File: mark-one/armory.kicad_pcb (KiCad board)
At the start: 8 copper layers, 65.6 x 19.6 mm, 184 parts, among them J1 MICRO_SD_HINGE, J2 USB_A_PLUG, P1 TST, P10 TST, P11 TST, P12 TST, P13 TST, P2 TST, P3 TST, P4 CONN_01X07, P5 TST, P6 TST, P8 TST, P9 TST, U2 MX53, U3 NCP1529, U4 MT41K256M16HA, U5 TPD2E001DRLR, X1 32.768kHz, X2 24MHz

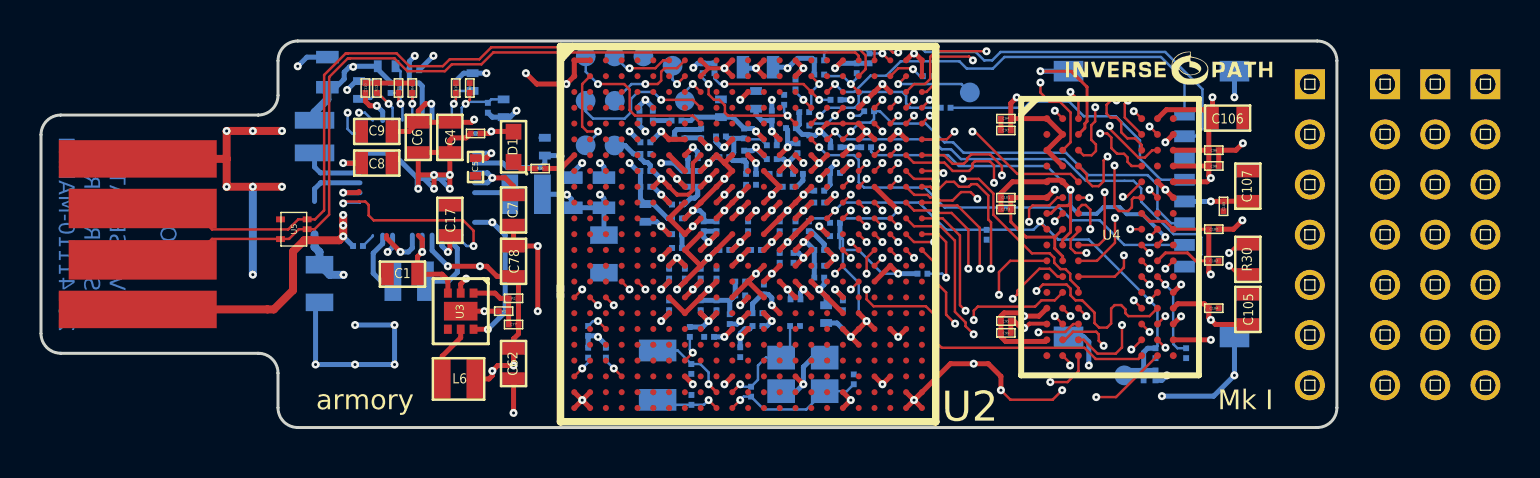
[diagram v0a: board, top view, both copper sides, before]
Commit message: added zones again
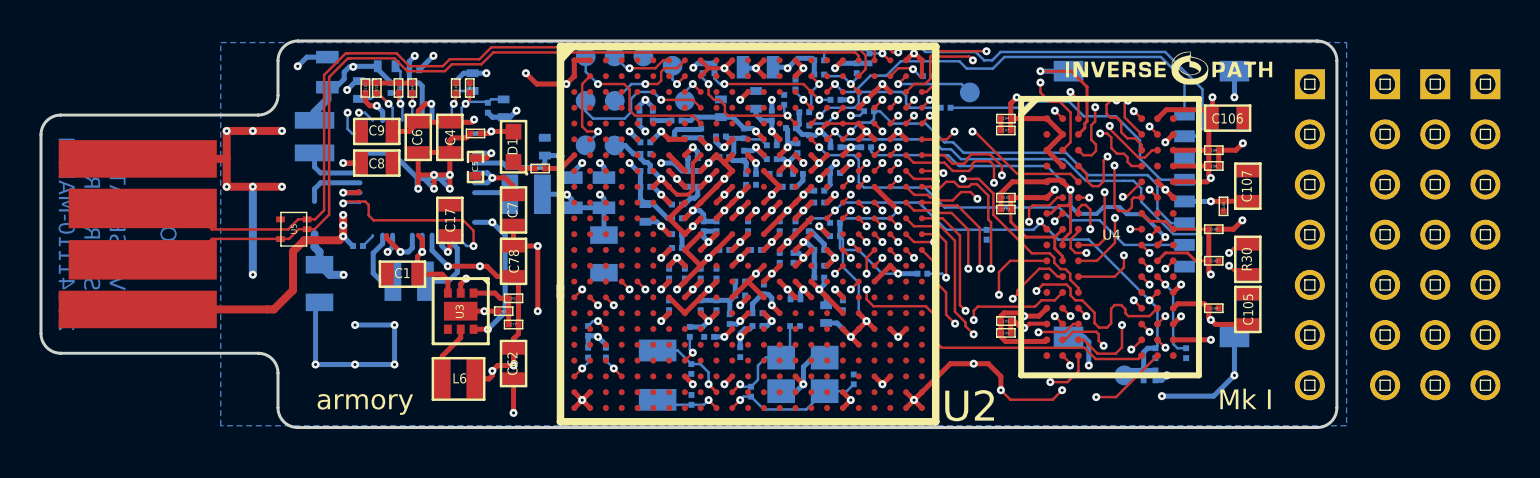
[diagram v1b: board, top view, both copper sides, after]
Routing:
- added copper zone on GND_POWER_2, net /Interfaces/USB_VBUS
- added copper zone on B.Cu, net GND
- added copper zone on SIGNAL_2, net GND
- added copper zone on GND_POWER_1, net IMX53_LDO_1V8
- added copper zone on GND_POWER_2, net PMIC_DDR_1V5
- added copper zone on GND_POWER_1, net PMIC_LDO1_STDBY
- added copper zone on GND_POWER_2, net PMIC_SW1_VDDGP
- added copper zone on GND_POWER_1, net PMIC_SW2_VCC
- added copper zone on GND_POWER_1, net PMIC_SW3_2V5
- added copper zone on GND_POWER_2, net PMIC_SW4_3V3
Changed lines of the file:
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@@
   (layers
     (0 TOP signal)
-    (1 GND_1 power)
+    (1 GND_1 power hide)
     (2 SIGNAL_1 signal)
-    (3 GND_POWER_1 power)
-    (4 GND_POWER_2 power)
-    (5 SIGNAL_2 signal)
-    (6 GND_2 power)
-    (31 BOTTOM signal)
+    (3 GND_POWER_1 power hide)
+    (4 GND_POWER_2 power hide)
+    (5 SIGNAL_2 signal hide)
+    (6 GND_2 power hide)
+    (31 BOTTOM signal hide)
     (32 B.Adhes user)
     (33 F.Adhes user)
@@
   (segment (start 130.425 92.075) (end 129.625 92.075) (width 0.254) (layer TOP) (net 126))
   (segment (start 131.1 91.4) (end 130.425 92.075) (width 0.254) (layer TOP) (net 126))
+  (zone (net 1) (net_name GND) (layer BOTTOM) (hatch edge 0.508)
+    (connect_pads (clearance 0.25))
+    (min_thickness 0.127)
+    (fill (arc_segments 16) (thermal_gap 0.254) (thermal_bridge_width 0.4064))
+    (polygon
+      (pts
+        (xy 170.2 105.1) (xy 113.2 105.1) (xy 113.2 85.7) (xy 170.2 85.7)
+      )
+    )
+  )
+  (zone (net 1) (net_name GND) (layer SIGNAL_2) (hatch edge 0.508)
+    (connect_pads (clearance 0.127))
+    (min_thickness 0.127)
+    (fill (arc_segments 16) (thermal_gap 0.254) (thermal_bridge_width 0.4064))
+    (polygon
+      (pts
+        (xy 170.2 105.1) (xy 104 105.1) (xy 104 85.7) (xy 170.2 85.7)
+      )
+    )
+  )
+  (zone (net 55) (net_name PMIC_SW4_3V3) (layer GND_POWER_2) (hatch edge 0.508)
+    (connect_pads (clearance 0.127))
+    (min_thickness 0.127)
+    (fill (arc_segments 16) (thermal_gap 0.254) (thermal_bridge_width 0.4064))
+    (polygon
+      (pts
+        (xy 139.7 99.2) (xy 138.7 99.2) (xy 138.7 100.1) (xy 133.1 100.1) (xy 133.1 101)
+        (xy 131.4 101) (xy 117.45 101) (xy 117.45 88.6) (xy 121.3 88.6) (xy 121.3 90.75)
+        (xy 118.4 90.75) (xy 118.4 96.05) (xy 122.6 96.05) (xy 122.6 99) (xy 125 99)
+        (xy 130.725 99) (xy 130.725 97.6) (xy 135.2 97.6) (xy 135.2 96.3) (xy 135.8 96.3)
+        (xy 135.8 98.7) (xy 139.7 98.7)
+      )
+    )
+  )
+  (zone (net 59) (net_name PMIC_DDR_1V5) (layer GND_POWER_2) (hatch edge 0.508)
+    (connect_pads (clearance 0.127))
+    (min_thickness 0.127)
+    (fill (arc_segments 16) (thermal_gap 0.254) (thermal_bridge_width 0.4064))
+    (polygon
+      (pts
+        (xy 146.45 104.05) (xy 124.6 104.05) (xy 124.6 101.85) (xy 144.1 101.85) (xy 144.1 92.5)
+        (xy 144.8 92.5) (xy 144.8 91.5) (xy 144.8 88.23) (xy 164.05 88.23) (xy 164.05 104.05)
+      )
+    )
+  )
+  (zone (net 58) (net_name PMIC_SW2_VCC) (layer GND_POWER_1) (hatch edge 0.508)
+    (connect_pads (clearance 0.127))
+    (min_thickness 0.127)
+    (fill (arc_segments 16) (thermal_gap 0.254) (thermal_bridge_width 0.4064))
+    (polygon
+      (pts
+        (xy 143.9 98.5) (xy 136 98.5) (xy 136 97.8) (xy 119.1 97.8) (xy 119.1 94.45)
+        (xy 119.7 94.45) (xy 119.7 91.05) (xy 118.775 91.05) (xy 118.775 87.65) (xy 119.95 87.65)
+        (xy 119.95 88.1) (xy 120.35 88.1) (xy 120.35 93.6) (xy 120.2 93.6) (xy 120.2 96.5)
+        (xy 119.75 96.5) (xy 119.75 97) (xy 123.05 97) (xy 123.05 96.525) (xy 124.35 96.525)
+        (xy 124.35 95.2) (xy 125.3 95.2) (xy 125.3 97) (xy 136 97) (xy 136 96.3)
+        (xy 140.8 96.3) (xy 140.8 93.2) (xy 143 93.2) (xy 143 97.4) (xy 143.9 97.4)
+        (xy 143.9 98.5)
+      )
+    )
+  )
+  (zone (net 60) (net_name IMX53_LDO_1V8) (layer GND_POWER_1) (hatch edge 0.508)
+    (connect_pads (clearance 0.127))
+    (min_thickness 0.127)
+    (fill (arc_segments 16) (thermal_gap 0.254) (thermal_bridge_width 0.4064))
+    (polygon
+      (pts
+        (xy 143.7 92.75) (xy 140.3 92.75) (xy 140.3 95.35) (xy 125.8 95.35) (xy 125.8 94.7)
+        (xy 122.1 94.7) (xy 122.1 96.5) (xy 120.7 96.5) (xy 120.7 94.1) (xy 125.8 94.1)
+        (xy 125.8 93.25) (xy 138.7 93.25) (xy 138.7 92.5) (xy 142.6 92.5) (xy 142.6 91.6)
+        (xy 143.7 91.6)
+      )
+    )
+  )
   (zone (net 54) (net_name PMIC_LDO3_2V8) (layer GND_POWER_1) (hatch edge 0.508)
     (connect_pads (clearance 0.127))
@@
     )
   )
+  (zone (net 53) (net_name PMIC_LDO1_STDBY) (layer GND_POWER_1) (hatch edge 0.508)
+    (connect_pads (clearance 0.127))
+    (min_thickness 0.127)
+    (fill (arc_segments 16) (thermal_gap 0.254) (thermal_bridge_width 0.4064))
+    (polygon
+      (pts
+        (xy 138.925 100.9) (xy 133.3 100.9) (xy 133.3 101.9) (xy 131.1 101.9) (xy 117.4 101.9)
+        (xy 117.4 85.75) (xy 123.25 85.75) (xy 123.25 86.65) (xy 122.8 86.65) (xy 122.8 86.2)
+        (xy 118.3 86.2) (xy 118.3 100.3) (xy 138.925 100.3)
+      )
+    )
+  )
   (zone (net 110) (net_name IMX53_LDO_1V3) (layer GND_POWER_2) (hatch edge 0.508)
     (connect_pads (clearance 0.127))
@@
     )
   )
+  (zone (net 119) (net_name /Interfaces/USB_VBUS) (layer GND_POWER_2) (hatch edge 0.508)
+    (connect_pads (clearance 0.127))
+    (min_thickness 0.127)
+    (fill (arc_segments 16) (thermal_gap 0.127) (thermal_bridge_width 0.4064))
+    (polygon
+      (pts
+        (xy 169.4 91.4) (xy 166.15 91.4) (xy 166.15 87.75) (xy 144.8 87.75) (xy 144.8 86.4)
+        (xy 138.425 86.4) (xy 138.425 87.4) (xy 136.8 87.4) (xy 136.8 86.4) (xy 125.3 86.4)
+        (xy 125.3 88.225) (xy 127.2 88.225) (xy 127.2 90.55) (xy 126.25 90.55) (xy 126.25 92)
+        (xy 127.2 92) (xy 127.2 94.1) (xy 124.2 94.1) (xy 124.2 96.6) (xy 123.175 96.6)
+        (xy 123.175 95.575) (xy 119.1 95.575) (xy 119.1 95.075) (xy 119.1 91.4) (xy 123 91.4)
+        (xy 123 85.8) (xy 169.4 85.8)
+      )
+    )
+  )
+  (zone (net 57) (net_name PMIC_SW1_VDDGP) (layer GND_POWER_2) (hatch edge 0.508)
+    (connect_pads (clearance 0.127))
+    (min_thickness 0.254)
+    (fill (arc_segments 16) (thermal_gap 0.508) (thermal_bridge_width 0.508))
+    (polygon
+      (pts
+        (xy 140.6 94.4) (xy 129.675 94.4) (xy 129.675 88.3) (xy 127.8 88.3) (xy 127.8 87.725)
+        (xy 126.375 87.725) (xy 126.375 86.9) (xy 130.825 86.9) (xy 130.825 90.7) (xy 137.3 90.7)
+        (xy 137.3 91.6) (xy 138.95 91.6) (xy 138.95 93.1) (xy 140.6 93.1)
+      )
+    )
+  )
   (zone (net 60) (net_name IMX53_LDO_1V8) (layer GND_POWER_2) (hatch edge 0.508)
     (connect_pads (clearance 0.127))
@@
       )
     )
+  )
+  (zone (net 56) (net_name PMIC_SW3_2V5) (layer GND_POWER_1) (hatch edge 0.508)
+    (connect_pads (clearance 0.127))
+    (min_thickness 0.127)
+    (fill (arc_segments 16) (thermal_gap 0.254) (thermal_bridge_width 0.4064))
+    (polygon
+      (pts
+        (xy 146.7 100.9) (xy 140.875 100.9) (xy 140.875 99.35) (xy 144.5 99.35) (xy 144.5 90.5)
+        (xy 145.9 90.5) (xy 145.9 87.9) (xy 135.9 87.9) (xy 135.9 89.2) (xy 133.5 89.2)
+        (xy 133.5 87.9) (xy 120.85 87.9) (xy 120.85 87.3) (xy 119.6 87.3) (xy 119.6 86.7)
+        (xy 122.2 86.7) (xy 122.2 87.15) (xy 123.9 87.15) (xy 123.9 85.75) (xy 146.7 85.75)
+      )
+    )
+  )
+  (zone (net 55) (net_name PMIC_SW4_3V3) (layer GND_POWER_1) (hatch edge 0.508)
+    (connect_pads (clearance 0.127))
+    (min_thickness 0.127)
+    (fill (arc_segments 16) (thermal_gap 0.254) (thermal_bridge_width 0.4064))
+    (polygon
+      (pts
+        (xy 164.125 104.875) (xy 139.725 104.875) (xy 139.725 99.5) (xy 139.275 99.5) (xy 139.275 98.775)
+        (xy 140.3 98.775) (xy 140.3 103.875) (xy 163.275 103.875) (xy 163.275 94.3) (xy 161.675 94.3)
+        (xy 161.675 93.275) (xy 164.125 93.275)
+      )
+    )
+  )
+  (zone (net 1) (net_name GND) (layer GND_POWER_1) (hatch edge 0.508)
+    (connect_pads (clearance 0.127))
+    (min_thickness 0.127)
+    (fill (arc_segments 16) (thermal_gap 0.254) (thermal_bridge_width 0.4064))
+    (polygon
+      (pts
+        (xy 164.625 92.775) (xy 161.175 92.775) (xy 161.175 94.8) (xy 162.775 94.8) (xy 162.775 103.375)
+        (xy 147.2 103.375) (xy 147.2 85.75) (xy 164.625 85.75)
+      )
+    )
+  )
+  (zone (net 59) (net_name PMIC_DDR_1V5) (layer GND_POWER_2) (hatch edge 0.508)
+    (connect_pads (clearance 0.127))
+    (min_thickness 0.127)
+    (fill (arc_segments 16) (thermal_gap 0.254) (thermal_bridge_width 0.4064))
+    (polygon
+      (pts
+        (xy 129.675 98.5) (xy 125.975 98.5) (xy 125.975 96.325) (xy 126.925 96.325) (xy 126.925 94.975)
+        (xy 127.75 94.975) (xy 127.75 89.65) (xy 129.175 89.65) (xy 129.175 94.975) (xy 129.675 94.975)
+      )
+    )

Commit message: removed zones
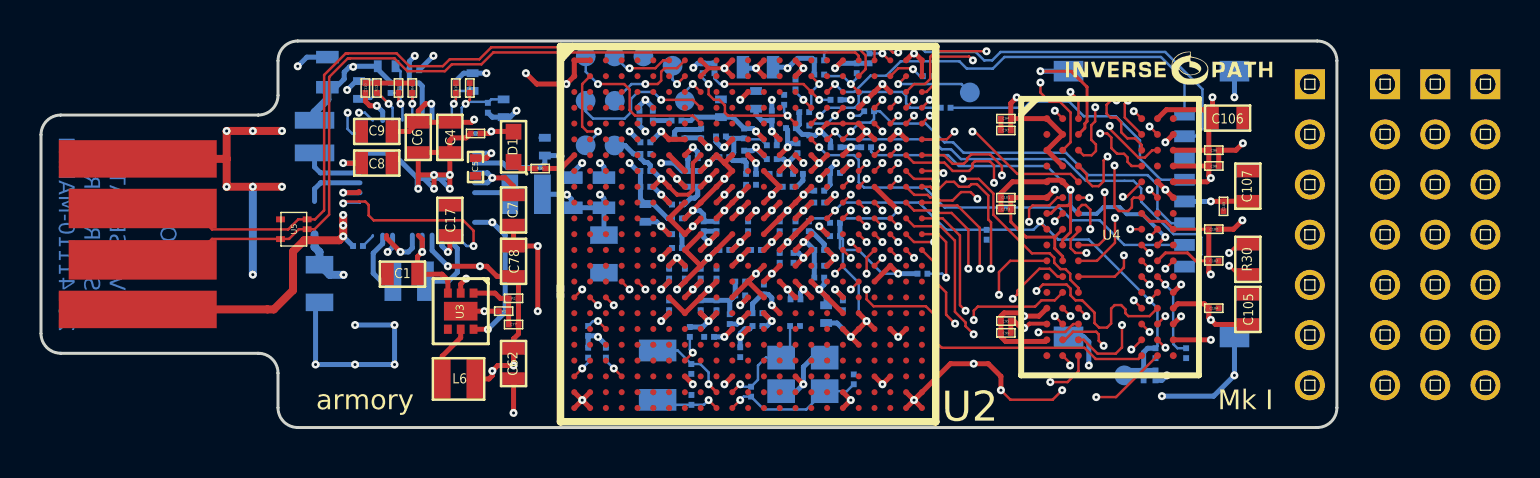
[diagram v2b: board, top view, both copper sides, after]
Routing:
- removed copper zone on GND_POWER_2, net /Interfaces/USB_VBUS
- removed copper zone on B.Cu, net GND
- removed copper zone on SIGNAL_2, net GND
- removed copper zone on GND_POWER_1, net IMX53_LDO_1V8
- removed copper zone on GND_POWER_2, net PMIC_DDR_1V5
- removed copper zone on GND_POWER_1, net PMIC_LDO1_STDBY
- removed copper zone on GND_POWER_2, net PMIC_SW1_VDDGP
- removed copper zone on GND_POWER_1, net PMIC_SW2_VCC
- removed copper zone on GND_POWER_1, net PMIC_SW3_2V5
- removed copper zone on GND_POWER_2, net PMIC_SW4_3V3
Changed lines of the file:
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@@
   (layers
     (0 TOP signal)
-    (1 GND_1 power hide)
+    (1 GND_1 power)
     (2 SIGNAL_1 signal)
-    (3 GND_POWER_1 power hide)
-    (4 GND_POWER_2 power hide)
-    (5 SIGNAL_2 signal hide)
-    (6 GND_2 power hide)
-    (31 BOTTOM signal hide)
+    (3 GND_POWER_1 power)
+    (4 GND_POWER_2 power)
+    (5 SIGNAL_2 signal)
+    (6 GND_2 power)
+    (31 BOTTOM signal)
     (32 B.Adhes user)
     (33 F.Adhes user)
@@
   (segment (start 130.425 92.075) (end 129.625 92.075) (width 0.254) (layer TOP) (net 126))
   (segment (start 131.1 91.4) (end 130.425 92.075) (width 0.254) (layer TOP) (net 126))
-  (zone (net 1) (net_name GND) (layer BOTTOM) (hatch edge 0.508)
-    (connect_pads (clearance 0.25))
-    (min_thickness 0.127)
-    (fill (arc_segments 16) (thermal_gap 0.254) (thermal_bridge_width 0.4064))
-    (polygon
-      (pts
-        (xy 170.2 105.1) (xy 113.2 105.1) (xy 113.2 85.7) (xy 170.2 85.7)
-      )
-    )
-  )
-  (zone (net 1) (net_name GND) (layer SIGNAL_2) (hatch edge 0.508)
-    (connect_pads (clearance 0.127))
-    (min_thickness 0.127)
-    (fill (arc_segments 16) (thermal_gap 0.254) (thermal_bridge_width 0.4064))
-    (polygon
-      (pts
-        (xy 170.2 105.1) (xy 104 105.1) (xy 104 85.7) (xy 170.2 85.7)
-      )
-    )
-  )
-  (zone (net 55) (net_name PMIC_SW4_3V3) (layer GND_POWER_2) (hatch edge 0.508)
-    (connect_pads (clearance 0.127))
-    (min_thickness 0.127)
-    (fill (arc_segments 16) (thermal_gap 0.254) (thermal_bridge_width 0.4064))
-    (polygon
-      (pts
-        (xy 139.7 99.2) (xy 138.7 99.2) (xy 138.7 100.1) (xy 133.1 100.1) (xy 133.1 101)
-        (xy 131.4 101) (xy 117.45 101) (xy 117.45 88.6) (xy 121.3 88.6) (xy 121.3 90.75)
-        (xy 118.4 90.75) (xy 118.4 96.05) (xy 122.6 96.05) (xy 122.6 99) (xy 125 99)
-        (xy 130.725 99) (xy 130.725 97.6) (xy 135.2 97.6) (xy 135.2 96.3) (xy 135.8 96.3)
-        (xy 135.8 98.7) (xy 139.7 98.7)
-      )
-    )
-  )
-  (zone (net 59) (net_name PMIC_DDR_1V5) (layer GND_POWER_2) (hatch edge 0.508)
-    (connect_pads (clearance 0.127))
-    (min_thickness 0.127)
-    (fill (arc_segments 16) (thermal_gap 0.254) (thermal_bridge_width 0.4064))
-    (polygon
-      (pts
-        (xy 146.45 104.05) (xy 124.6 104.05) (xy 124.6 101.85) (xy 144.1 101.85) (xy 144.1 92.5)
-        (xy 144.8 92.5) (xy 144.8 91.5) (xy 144.8 88.23) (xy 164.05 88.23) (xy 164.05 104.05)
-      )
-    )
-  )
-  (zone (net 58) (net_name PMIC_SW2_VCC) (layer GND_POWER_1) (hatch edge 0.508)
-    (connect_pads (clearance 0.127))
-    (min_thickness 0.127)
-    (fill (arc_segments 16) (thermal_gap 0.254) (thermal_bridge_width 0.4064))
-    (polygon
-      (pts
-        (xy 143.9 98.5) (xy 136 98.5) (xy 136 97.8) (xy 119.1 97.8) (xy 119.1 94.45)
-        (xy 119.7 94.45) (xy 119.7 91.05) (xy 118.775 91.05) (xy 118.775 87.65) (xy 119.95 87.65)
-        (xy 119.95 88.1) (xy 120.35 88.1) (xy 120.35 93.6) (xy 120.2 93.6) (xy 120.2 96.5)
-        (xy 119.75 96.5) (xy 119.75 97) (xy 123.05 97) (xy 123.05 96.525) (xy 124.35 96.525)
-        (xy 124.35 95.2) (xy 125.3 95.2) (xy 125.3 97) (xy 136 97) (xy 136 96.3)
-        (xy 140.8 96.3) (xy 140.8 93.2) (xy 143 93.2) (xy 143 97.4) (xy 143.9 97.4)
-        (xy 143.9 98.5)
-      )
-    )
-  )
-  (zone (net 60) (net_name IMX53_LDO_1V8) (layer GND_POWER_1) (hatch edge 0.508)
-    (connect_pads (clearance 0.127))
-    (min_thickness 0.127)
-    (fill (arc_segments 16) (thermal_gap 0.254) (thermal_bridge_width 0.4064))
-    (polygon
-      (pts
-        (xy 143.7 92.75) (xy 140.3 92.75) (xy 140.3 95.35) (xy 125.8 95.35) (xy 125.8 94.7)
-        (xy 122.1 94.7) (xy 122.1 96.5) (xy 120.7 96.5) (xy 120.7 94.1) (xy 125.8 94.1)
-        (xy 125.8 93.25) (xy 138.7 93.25) (xy 138.7 92.5) (xy 142.6 92.5) (xy 142.6 91.6)
-        (xy 143.7 91.6)
-      )
-    )
-  )
   (zone (net 54) (net_name PMIC_LDO3_2V8) (layer GND_POWER_1) (hatch edge 0.508)
     (connect_pads (clearance 0.127))
@@
     )
   )
-  (zone (net 53) (net_name PMIC_LDO1_STDBY) (layer GND_POWER_1) (hatch edge 0.508)
-    (connect_pads (clearance 0.127))
-    (min_thickness 0.127)
-    (fill (arc_segments 16) (thermal_gap 0.254) (thermal_bridge_width 0.4064))
-    (polygon
-      (pts
-        (xy 138.925 100.9) (xy 133.3 100.9) (xy 133.3 101.9) (xy 131.1 101.9) (xy 117.4 101.9)
-        (xy 117.4 85.75) (xy 123.25 85.75) (xy 123.25 86.65) (xy 122.8 86.65) (xy 122.8 86.2)
-        (xy 118.3 86.2) (xy 118.3 100.3) (xy 138.925 100.3)
-      )
-    )
-  )
   (zone (net 110) (net_name IMX53_LDO_1V3) (layer GND_POWER_2) (hatch edge 0.508)
     (connect_pads (clearance 0.127))
@@
     )
   )
-  (zone (net 119) (net_name /Interfaces/USB_VBUS) (layer GND_POWER_2) (hatch edge 0.508)
-    (connect_pads (clearance 0.127))
-    (min_thickness 0.127)
-    (fill (arc_segments 16) (thermal_gap 0.127) (thermal_bridge_width 0.4064))
-    (polygon
-      (pts
-        (xy 169.4 91.4) (xy 166.15 91.4) (xy 166.15 87.75) (xy 144.8 87.75) (xy 144.8 86.4)
-        (xy 138.425 86.4) (xy 138.425 87.4) (xy 136.8 87.4) (xy 136.8 86.4) (xy 125.3 86.4)
-        (xy 125.3 88.225) (xy 127.2 88.225) (xy 127.2 90.55) (xy 126.25 90.55) (xy 126.25 92)
-        (xy 127.2 92) (xy 127.2 94.1) (xy 124.2 94.1) (xy 124.2 96.6) (xy 123.175 96.6)
-        (xy 123.175 95.575) (xy 119.1 95.575) (xy 119.1 95.075) (xy 119.1 91.4) (xy 123 91.4)
-        (xy 123 85.8) (xy 169.4 85.8)
-      )
-    )
-  )
-  (zone (net 57) (net_name PMIC_SW1_VDDGP) (layer GND_POWER_2) (hatch edge 0.508)
-    (connect_pads (clearance 0.127))
-    (min_thickness 0.254)
-    (fill (arc_segments 16) (thermal_gap 0.508) (thermal_bridge_width 0.508))
-    (polygon
-      (pts
-        (xy 140.6 94.4) (xy 129.675 94.4) (xy 129.675 88.3) (xy 127.8 88.3) (xy 127.8 87.725)
-        (xy 126.375 87.725) (xy 126.375 86.9) (xy 130.825 86.9) (xy 130.825 90.7) (xy 137.3 90.7)
-        (xy 137.3 91.6) (xy 138.95 91.6) (xy 138.95 93.1) (xy 140.6 93.1)
-      )
-    )
-  )
   (zone (net 60) (net_name IMX53_LDO_1V8) (layer GND_POWER_2) (hatch edge 0.508)
     (connect_pads (clearance 0.127))
@@
       )
     )
-  )
-  (zone (net 56) (net_name PMIC_SW3_2V5) (layer GND_POWER_1) (hatch edge 0.508)
-    (connect_pads (clearance 0.127))
-    (min_thickness 0.127)
-    (fill (arc_segments 16) (thermal_gap 0.254) (thermal_bridge_width 0.4064))
-    (polygon
-      (pts
-        (xy 146.7 100.9) (xy 140.875 100.9) (xy 140.875 99.35) (xy 144.5 99.35) (xy 144.5 90.5)
-        (xy 145.9 90.5) (xy 145.9 87.9) (xy 135.9 87.9) (xy 135.9 89.2) (xy 133.5 89.2)
-        (xy 133.5 87.9) (xy 120.85 87.9) (xy 120.85 87.3) (xy 119.6 87.3) (xy 119.6 86.7)
-        (xy 122.2 86.7) (xy 122.2 87.15) (xy 123.9 87.15) (xy 123.9 85.75) (xy 146.7 85.75)
-      )
-    )
-  )
-  (zone (net 55) (net_name PMIC_SW4_3V3) (layer GND_POWER_1) (hatch edge 0.508)
-    (connect_pads (clearance 0.127))
-    (min_thickness 0.127)
-    (fill (arc_segments 16) (thermal_gap 0.254) (thermal_bridge_width 0.4064))
-    (polygon
-      (pts
-        (xy 164.125 104.875) (xy 139.725 104.875) (xy 139.725 99.5) (xy 139.275 99.5) (xy 139.275 98.775)
-        (xy 140.3 98.775) (xy 140.3 103.875) (xy 163.275 103.875) (xy 163.275 94.3) (xy 161.675 94.3)
-        (xy 161.675 93.275) (xy 164.125 93.275)
-      )
-    )
-  )
-  (zone (net 1) (net_name GND) (layer GND_POWER_1) (hatch edge 0.508)
-    (connect_pads (clearance 0.127))
-    (min_thickness 0.127)
-    (fill (arc_segments 16) (thermal_gap 0.254) (thermal_bridge_width 0.4064))
-    (polygon
-      (pts
-        (xy 164.625 92.775) (xy 161.175 92.775) (xy 161.175 94.8) (xy 162.775 94.8) (xy 162.775 103.375)
-        (xy 147.2 103.375) (xy 147.2 85.75) (xy 164.625 85.75)
-      )
-    )
-  )
-  (zone (net 59) (net_name PMIC_DDR_1V5) (layer GND_POWER_2) (hatch edge 0.508)
-    (connect_pads (clearance 0.127))
-    (min_thickness 0.127)
-    (fill (arc_segments 16) (thermal_gap 0.254) (thermal_bridge_width 0.4064))
-    (polygon
-      (pts
-        (xy 129.675 98.5) (xy 125.975 98.5) (xy 125.975 96.325) (xy 126.925 96.325) (xy 126.925 94.975)
-        (xy 127.75 94.975) (xy 127.75 89.65) (xy 129.175 89.65) (xy 129.175 94.975) (xy 129.675 94.975)
-      )
-    )
